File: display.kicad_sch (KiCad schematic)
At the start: 7 parts, among them J5 Oled SSD1306 128x32, J9 Adafruit ST7789, U6 SS1306_OLEDM0.91_1x-I2C

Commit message: Actualización de esquemas y PCB con datos LCSC y librerías JLC
- Añade propiedades LCSC a los símbolos de las hojas de esquema
- Actualiza las hojas TXS0108E, display, esp32_c6, ft232, inmp441,
  led_sw_gpio, max98357a, micro_sd, power_supply y el esquema raíz
- Reorganiza el PCB (footprints, jumpers y nets) y actualiza el proyecto
- Incluye las librerías locales JLCImport (símbolos, huellas y modelos 3D)
  y las entradas correspondientes en fp-lib-table y sym-lib-table
- Añade la documentación técnica en docs/ y el archivo de posiciones
  esp32_xiaozhi-all.pos
- Elimina los ZIP generados gebers.zip y production.zip
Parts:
- C27: LCSC (none) -> C1525
- C33: LCSC (none) -> C28323
- J5: LCSC (none) -> C9900045120
- J9: LCSC (none) -> C9900247203; now left out of the parts list
- R41, R42: LCSC (none) -> C4190
- U6: now left out of the parts list
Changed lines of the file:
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@@
+			)
+		)
+		(property "LCSC" "C1525"
+			(at 163.83 137.16 0)
+			(hide yes)
+			(show_name no)
+			(do_not_autoplace no)
+			(effects
+				(font
+					(size 1.27 1.27)
+				)
 			)
 		)
@@
 			)
 		)
+		(property "LCSC" "C9900045120"
+			(at 149.86 76.2 0)
+			(hide yes)
+			(show_name no)
+			(do_not_autoplace no)
+			(effects
+				(font
+					(size 1.27 1.27)
+				)
+			)
+		)
 		(pin "3"
 		)
@@
 		(body_style 1)
 		(exclude_from_sim no)
-		(in_bom yes)
-		(on_board yes)
-		(in_pos_files yes)
+		(in_bom no)
+		(on_board yes)
+		(in_pos_files no)
 		(dnp no)
 		(property "Reference" "J9"
@@
 		(property "Description" "Display LCD ST7789 240x240 pixels"
 			(at 208.534 112.776 0)
+			(show_name no)
+			(do_not_autoplace no)
+			(effects
+				(font
+					(size 1.27 1.27)
+				)
+			)
+		)
+		(property "LCSC" "C9900247203"
+			(at 195.58 101.6 0)
+			(hide yes)
 			(show_name no)
 			(do_not_autoplace no)
@@
 			)
 		)
+		(property "LCSC" "C28323  "
+			(at 177.8 137.16 0)
+			(hide yes)
+			(show_name no)
+			(do_not_autoplace no)
+			(effects
+				(font
+					(size 1.27 1.27)
+				)
+			)
+		)
 		(pin "1"
 		)
@@
 			)
 		)
+		(property "LCSC" "C4190"
+			(at 110.49 130.81 0)
+			(hide yes)
+			(show_name no)
+			(do_not_autoplace no)
+			(effects
+				(font
+					(size 1.27 1.27)
+				)
+			)
+		)
 		(pin "1"
 		)
@@
 			)
 		)
+		(property "LCSC" "C4190"
+			(at 96.52 120.65 0)
+			(hide yes)
+			(show_name no)
+			(do_not_autoplace no)
+			(effects
+				(font
+					(size 1.27 1.27)
+				)
+			)
+		)
 		(pin "1"
 		)
@@
 		(body_style 1)
 		(exclude_from_sim no)
-		(in_bom yes)
-		(on_board yes)
-		(in_pos_files yes)
+		(in_bom no)
+		(on_board yes)
+		(in_pos_files no)
 		(dnp no)
 		(fields_autoplaced yes)

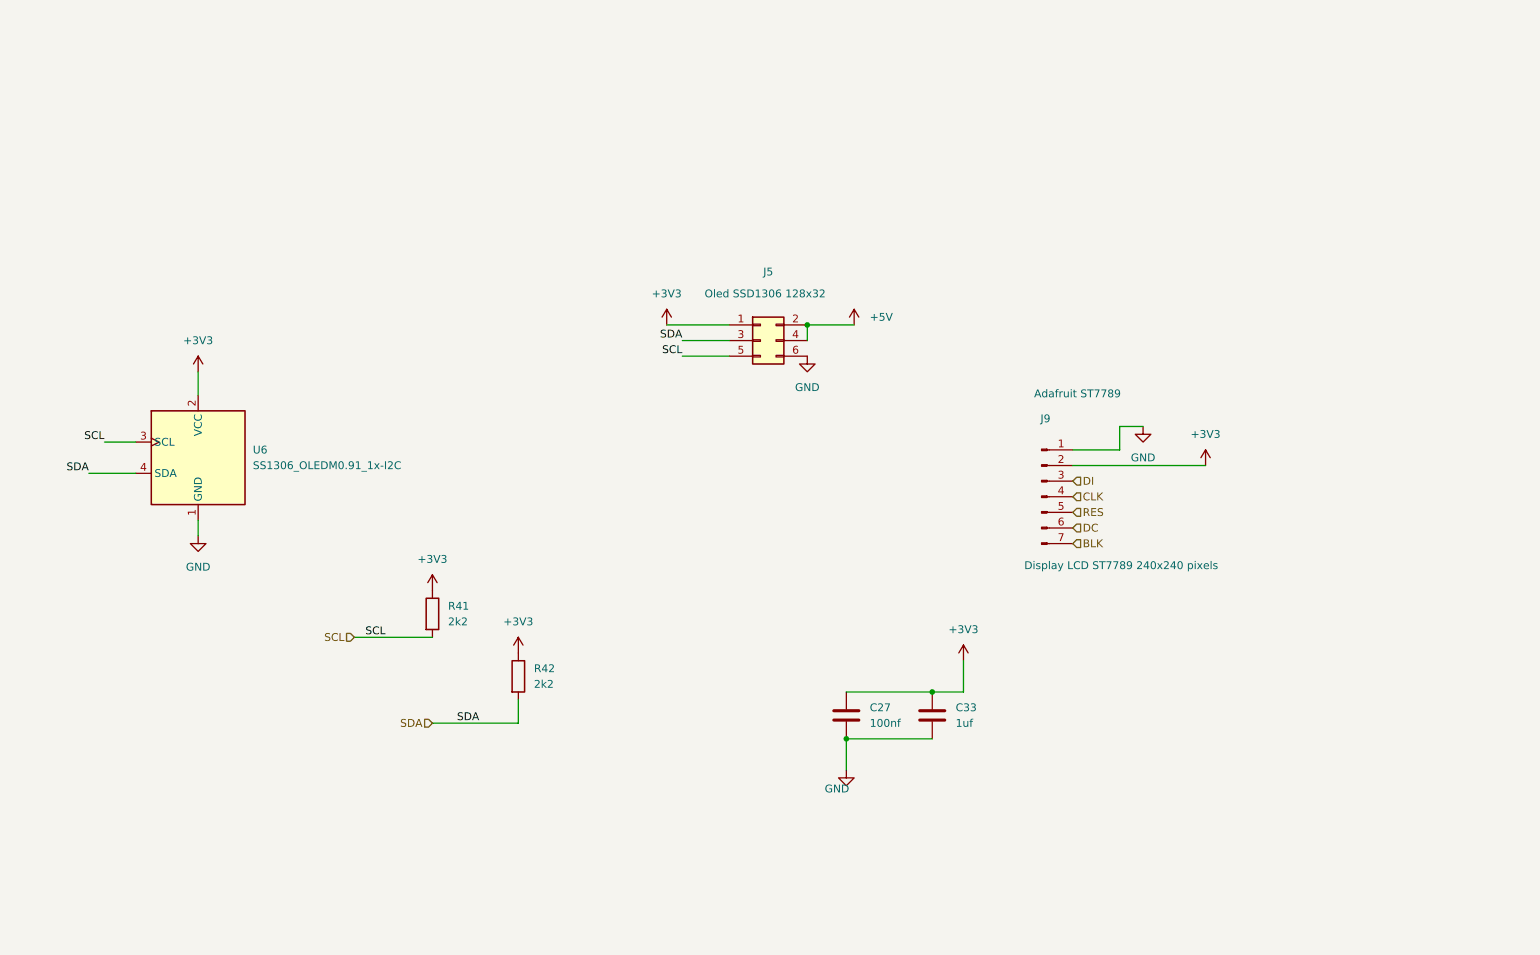
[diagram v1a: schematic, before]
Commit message: Actualización de esquemas, PCB y librerías
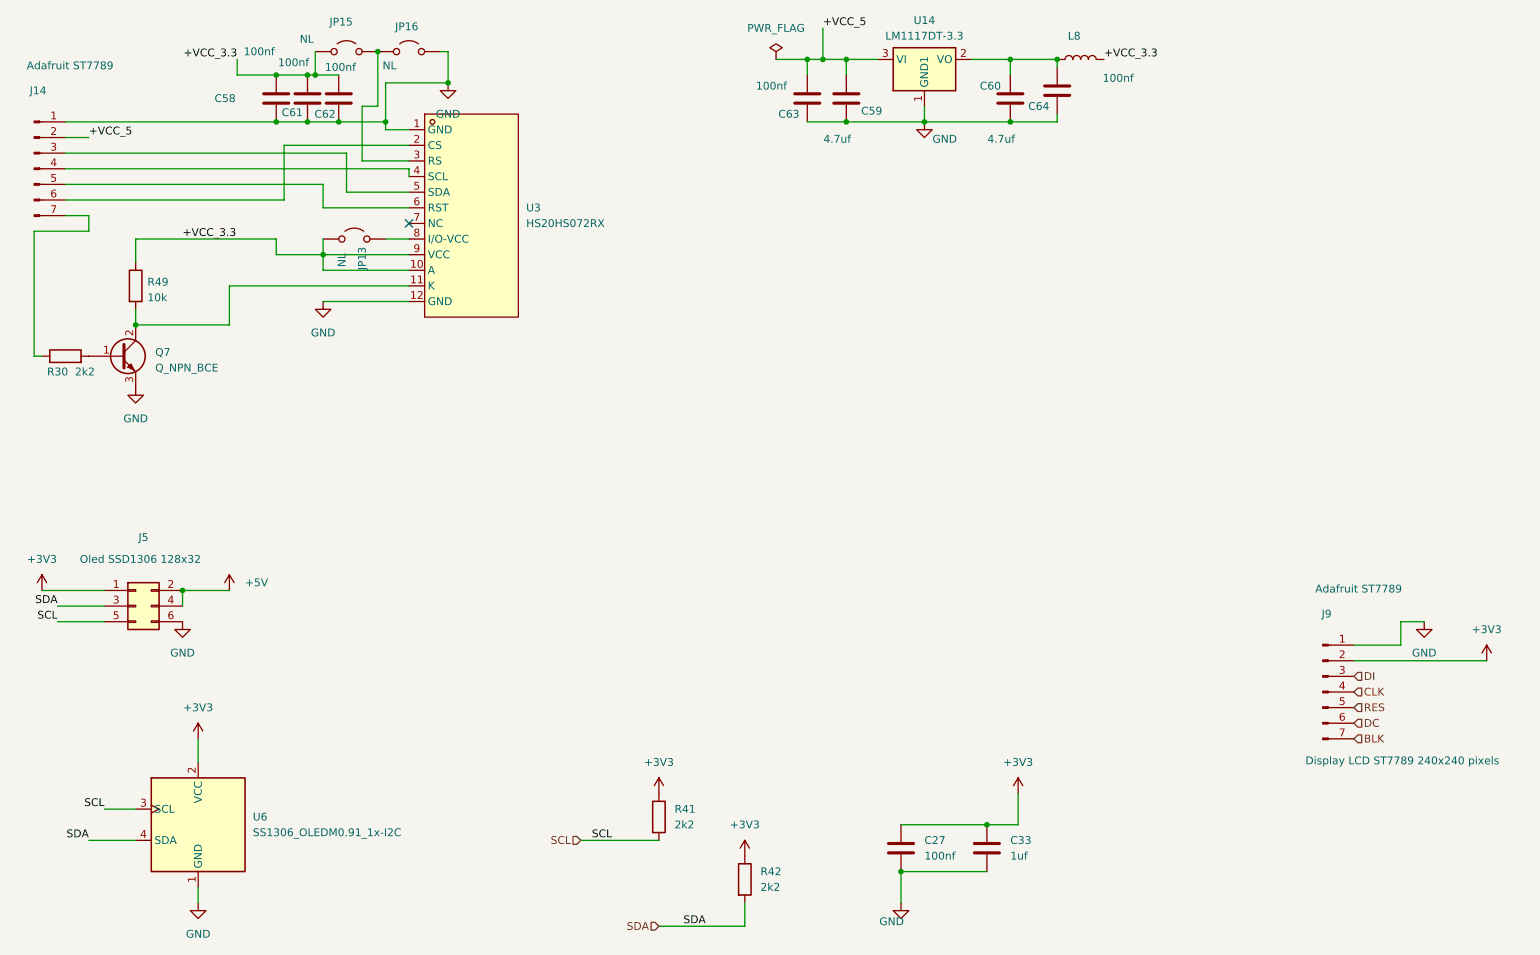
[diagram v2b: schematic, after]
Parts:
- added C58, C61, C62, C63, C64: 100nf, Capacitor_SMD:C_0402_1005Metric, symbol Device:C
- added C59, C60: 4.7uf, Capacitor_SMD:C_0805_2012Metric, symbol Device:C
- added J14: Adafruit ST7789, Connector_PinHeader_2.54mm:PinHeader_1x08_P2.54mm_Vertical, symbol Connector:Conn_01x07_Pin
- added JP13, JP15, JP16: NL, Jumper:SolderJumper-2_P1.3mm_Open_RoundedPad1.0x1.5mm, symbol Jumper:Jumper_2_Open
- added L8: 100mh, Inductor_SMD:L_1206_3216Metric, symbol Device:L
- added Q7: Q_NPN_BCE, Package_TO_SOT_SMD:SOT-23W, symbol Device:Q_NPN_BCE
- added R30: 2k2, Resistor_SMD:R_0805_2012Metric, symbol Device:R
- added R49: 10k, Resistor_SMD:R_0805_2012Metric, symbol Device:R
- added U14: LM1117DT-3.3, kiC:TO-252-3_TabPin2, symbol Regulator_Linear:LM1117DT-3.3
- added U3: HS20HS072RX, JLCImport:OLED-SMD_HS20HS072RX, symbol HS20HS072RX:HS20HS072RX
- C27: LCSC C1525 -> C28233
- R41, R42: LCSC C4190 -> C17520
- U6: LCSC (none) -> C5248080; now in the parts list
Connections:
- net GND: now also C58.1, C59.1, C60.1, C61.1, C62.1, C63.1, C64.1, J14.1 (Pin_1), JP16.2 (B), Q7.3 (E), U14.1 (GND1), U3.1 (GND), U3.12 (GND)
- new net: JP15.2 (B), JP16.1 (A), U3.3 (RS)
- new net: J14.3 (Pin_3), U3.5 (SDA)
- new net: J14.4 (Pin_4), U3.4 (SCL)
- new net: J14.5 (Pin_5), U3.6 (RST)
- new net: J14.6 (Pin_6), U3.2 (CS)
- new net: J14.7 (Pin_7), R30.1
- new net: Q7.2 (C), R49.2, U3.11 (K)
- new net: JP13.2 (B), U3.8 (I/O-VCC)
- new net: C60.2, C64.2, L8.1, U14.2 (VO)
- new net: Q7.1 (B), R30.2
- new net +VCC_3.3: C58.2, C61.2, C62.2, JP13.1 (A), JP15.1 (A), L8.2, R49.1, U3.10 (A), U3.9 (VCC)
- new net +VCC_5: C59.2, C63.2, J14.2 (Pin_2), U14.3 (VI)
- no-connect marks 0 -> 1
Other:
- moved on the sheet: C27, C33, J5, J9, R41, R42, U6
